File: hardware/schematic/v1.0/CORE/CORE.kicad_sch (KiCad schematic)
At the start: 55 parts, among them J1 Conn_01x03_Socket, J2 Conn_Coaxial, J3 Conn_Coaxial, J4 Conn_Coaxial, J5 Conn_Coaxial, M1 ZYNQ7010&7020, U1 TXS02612RTWR, U2 SP3232, U3 SD_Card

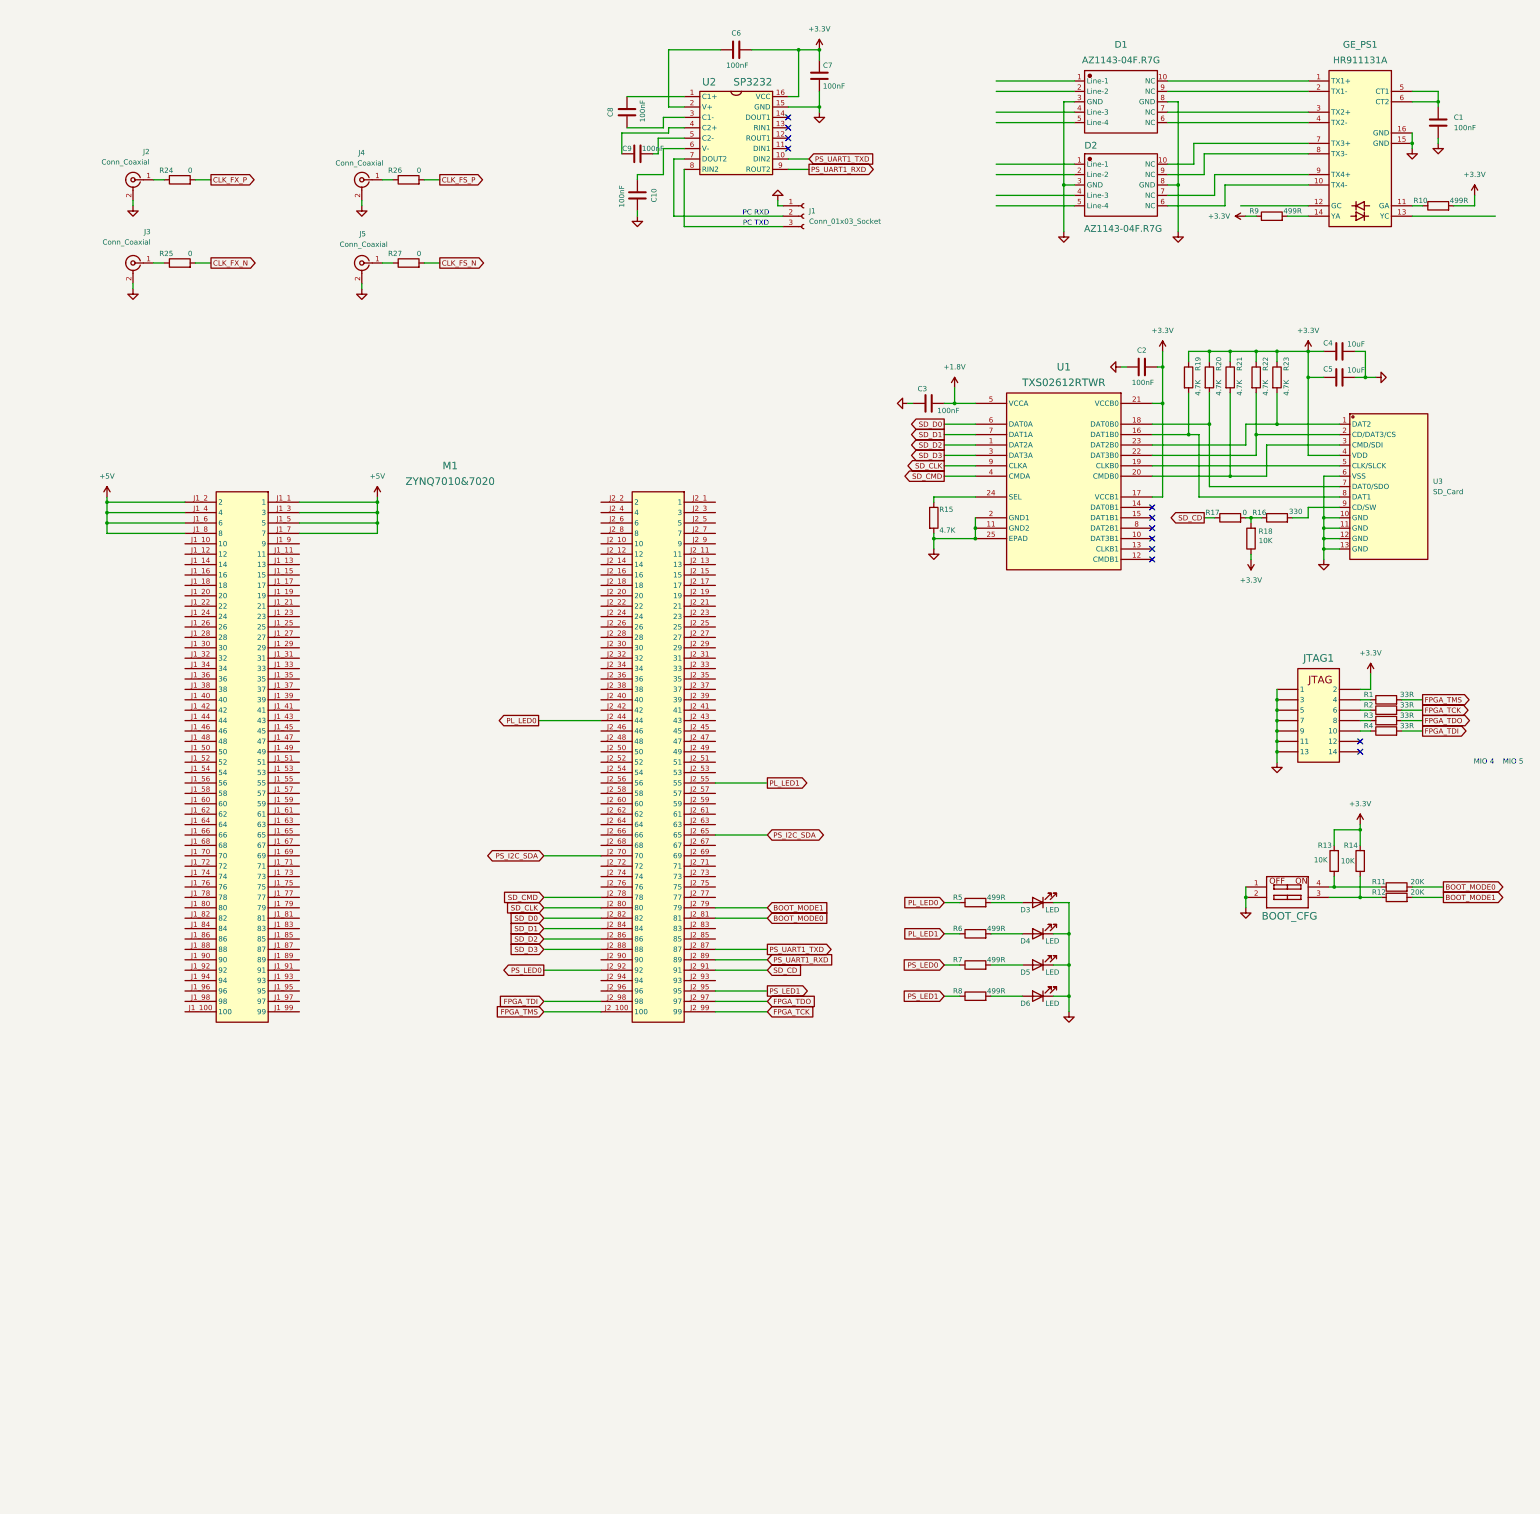
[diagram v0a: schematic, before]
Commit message: sch update
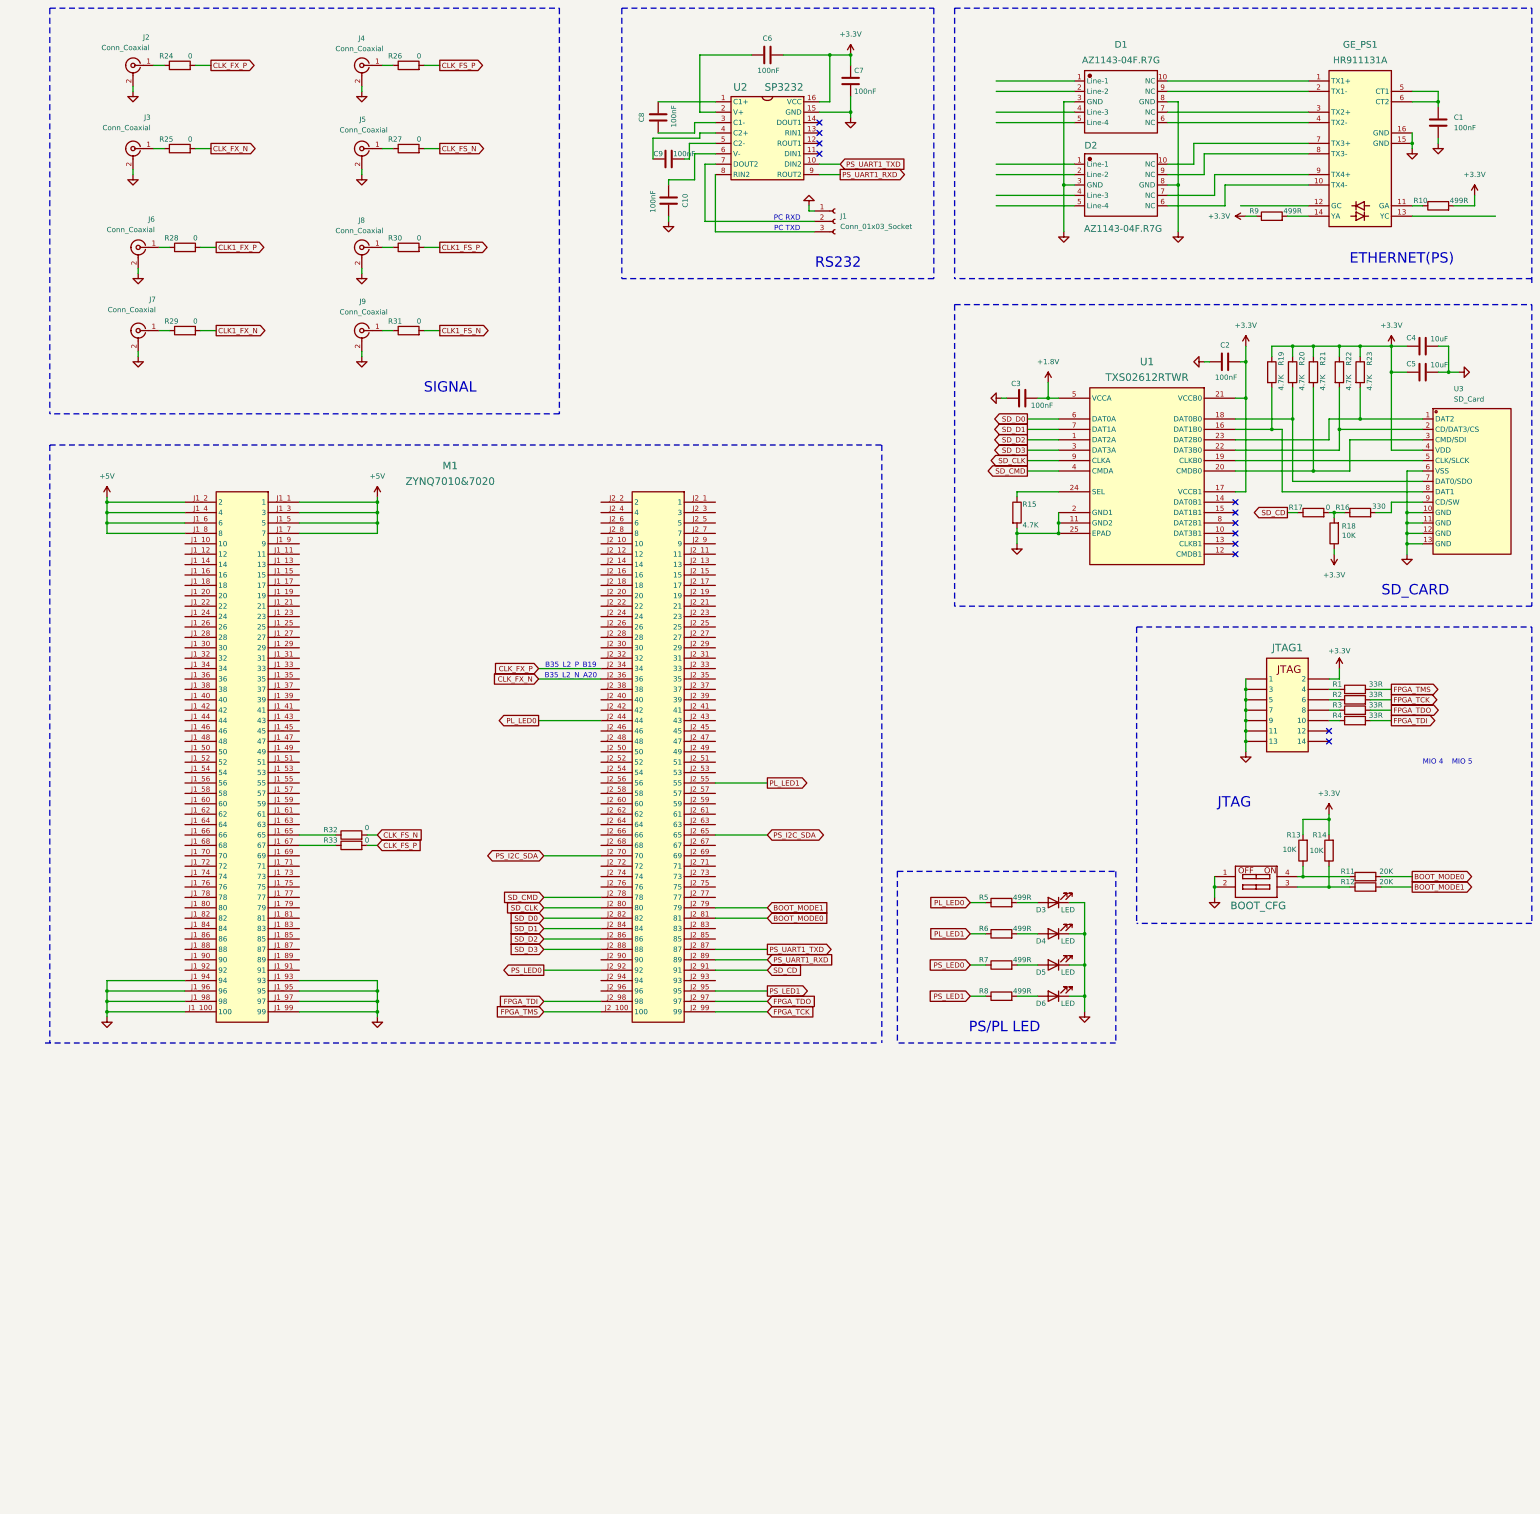
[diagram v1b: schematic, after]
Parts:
- added J6, J7, J8, J9: Conn_Coaxial, Connector_Coaxial:SMA_Amphenol_132289_EdgeMount, symbol Connector:Conn_Coaxial
- added R28, R29, R30, R31, R32, R33: 0, Resistor_SMD:R_0402_1005Metric, symbol Device:R
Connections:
- net CLK_FS_N: now also R32.2
- net CLK_FS_P: now also R33.2
- net CLK_FX_N: now also M1.J2_36 (36)
- net CLK_FX_P: now also M1.J2_34 (34)
- net GND: now also M1.J1_100 (100), M1.J1_93 (93), M1.J1_94 (94), M1.J1_95 (95), M1.J1_96 (96), M1.J1_97 (97), M1.J1_98 (98), M1.J1_99 (99), J6.2 (Ext), J7.2 (Ext), J8.2 (Ext), J9.2 (Ext)
- net at M1.J1_65 (65): now also R32.1
- net at M1.J1_67 (67): now also R33.1
- new net: J8.1 (In), R30.1
- new net: J7.1 (In), R29.1
- new net: J9.1 (In), R31.1
- new net: J6.1 (In), R28.1
- new net CLK1_FS_N: R31.2
- new net CLK1_FS_P: R30.2
- new net CLK1_FX_N: R29.2
- new net CLK1_FX_P: R28.2
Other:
- note added: "B35_L2_N_A20"
- note added: "B35_L2_P_B19"
- note added: "ETHERNET(PS)"
- note added: "JTAG"
- note added: "PS/PL LED"
- note added: "RS232"
- note added: "SD_CARD"
- note added: "SIGNAL"
- moved on the sheet: BOOT_CFG, C10, C2, C3, C4, C5, C6, C7, C8, C9, D3, D4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

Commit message: sch update
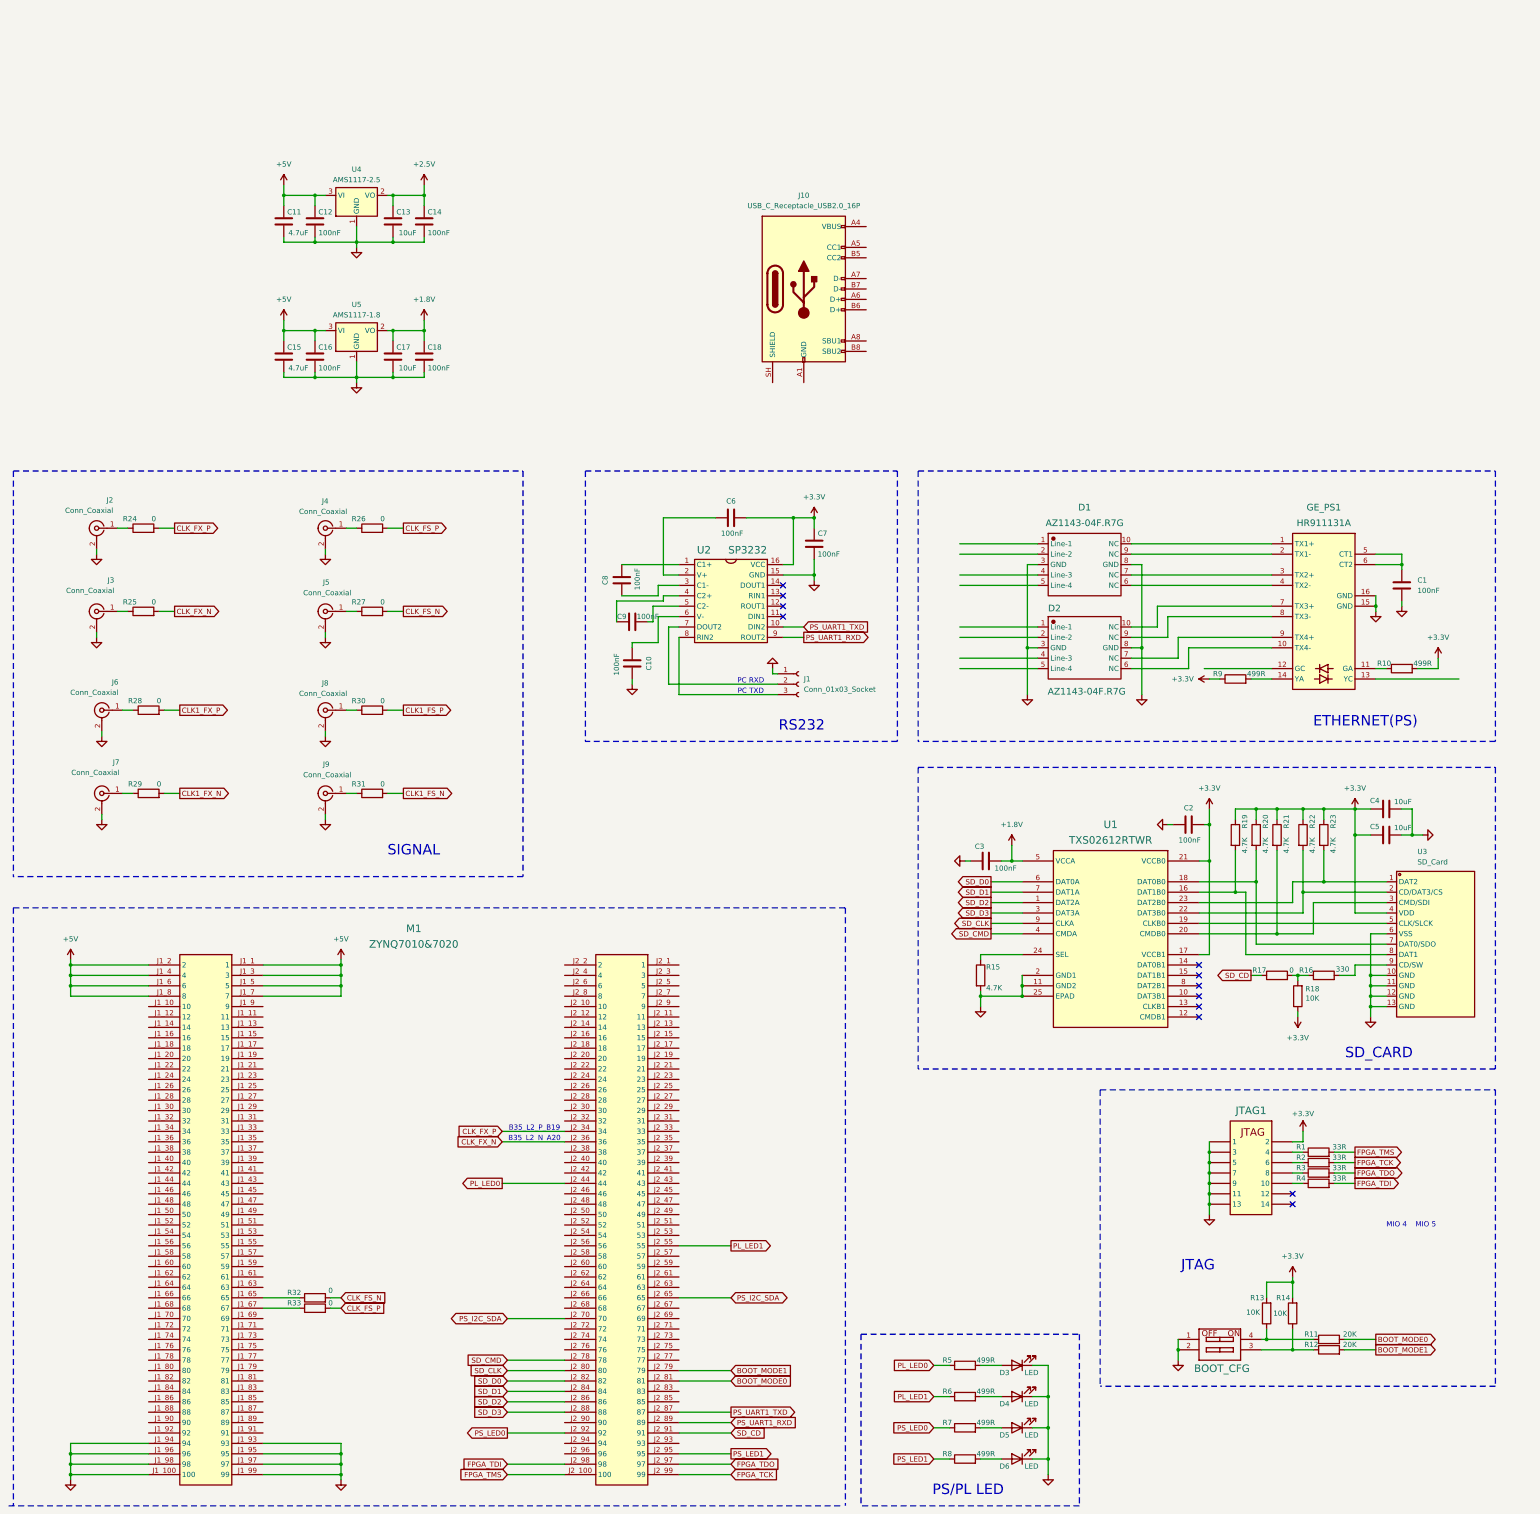
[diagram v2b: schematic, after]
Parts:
- added C11, C15: 4.7uF, Capacitor_SMD:C_0603_1608Metric, symbol Device:C
- added C12, C14, C16, C18: 100nF, Capacitor_SMD:C_0603_1608Metric, symbol Device:C
- added C13, C17: 10uF, Capacitor_SMD:C_0603_1608Metric, symbol Device:C
- added J10: USB_C_Receptacle_USB2.0_16P, symbol Connector:USB_C_Receptacle_USB2.0_16P
- added U4: AMS1117-2.5, Package_TO_SOT_SMD:SOT-223-3_TabPin2, symbol Regulator_Linear:AMS1117-2.5
- added U5: AMS1117-1.8, Package_TO_SOT_SMD:SOT-223-3_TabPin2, symbol Regulator_Linear:AMS1117-1.8
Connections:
- net +1.8V: now also C17.1, C18.1, U5.2 (VO)
- net +5V: now also C11.1, C12.1, C15.1, C16.1, U4.3 (VI), U5.3 (VI)
- net GND: now also C11.2, C12.2, C13.2, C14.2, C15.2, C16.2, C17.2, C18.2, U4.1 (GND), U5.1 (GND)
- new net: J10.A1 (GND), J10.A12 (GND), J10.B1 (GND), J10.B12 (GND)
- new net: J10.A4 (VBUS), J10.A9 (VBUS), J10.B4 (VBUS), J10.B9 (VBUS)
- new net +2.5V: C13.1, C14.1, U4.2 (VO)
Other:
- moved on the sheet: BOOT_CFG, C1, C10, C2, C3, C4, C5, C6, C7, C8, C9, D1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
